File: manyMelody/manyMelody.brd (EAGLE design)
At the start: 74.9 x 95.2 mm, 13 parts, among them IC1 788TV

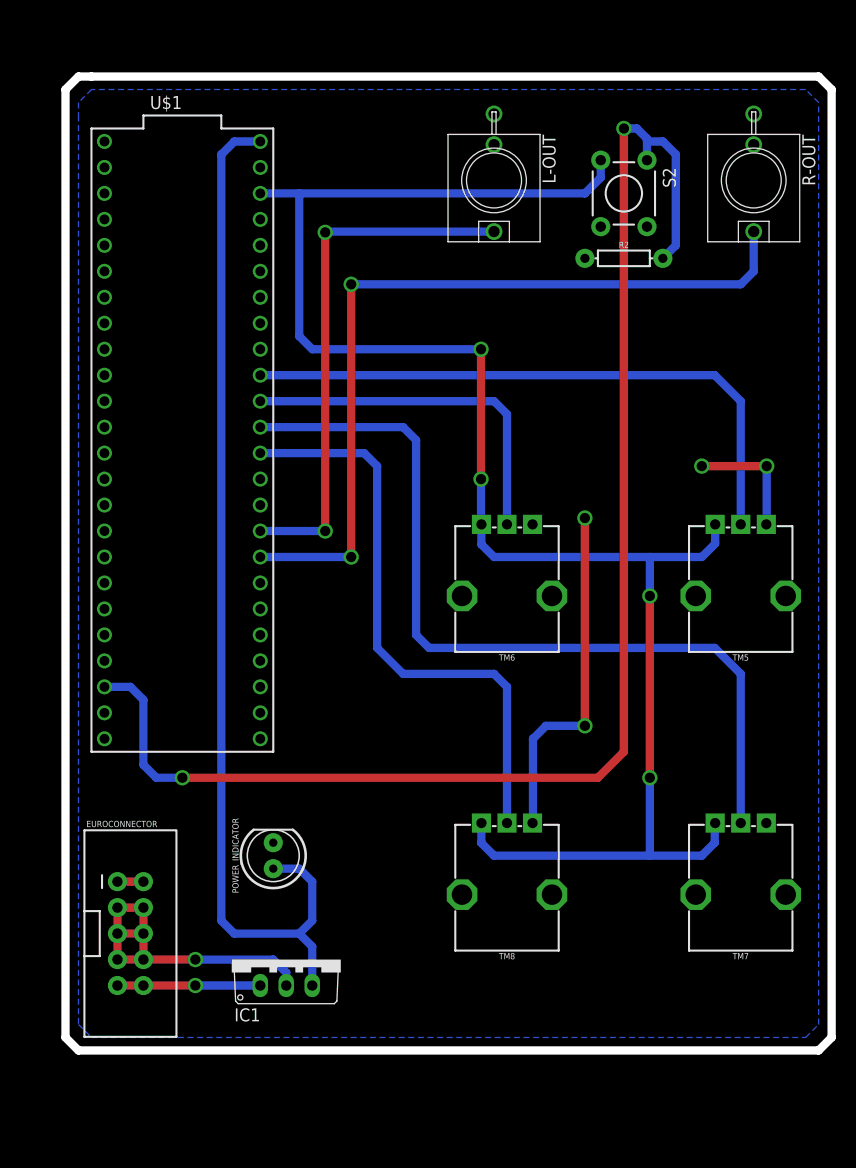
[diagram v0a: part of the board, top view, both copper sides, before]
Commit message: updated README
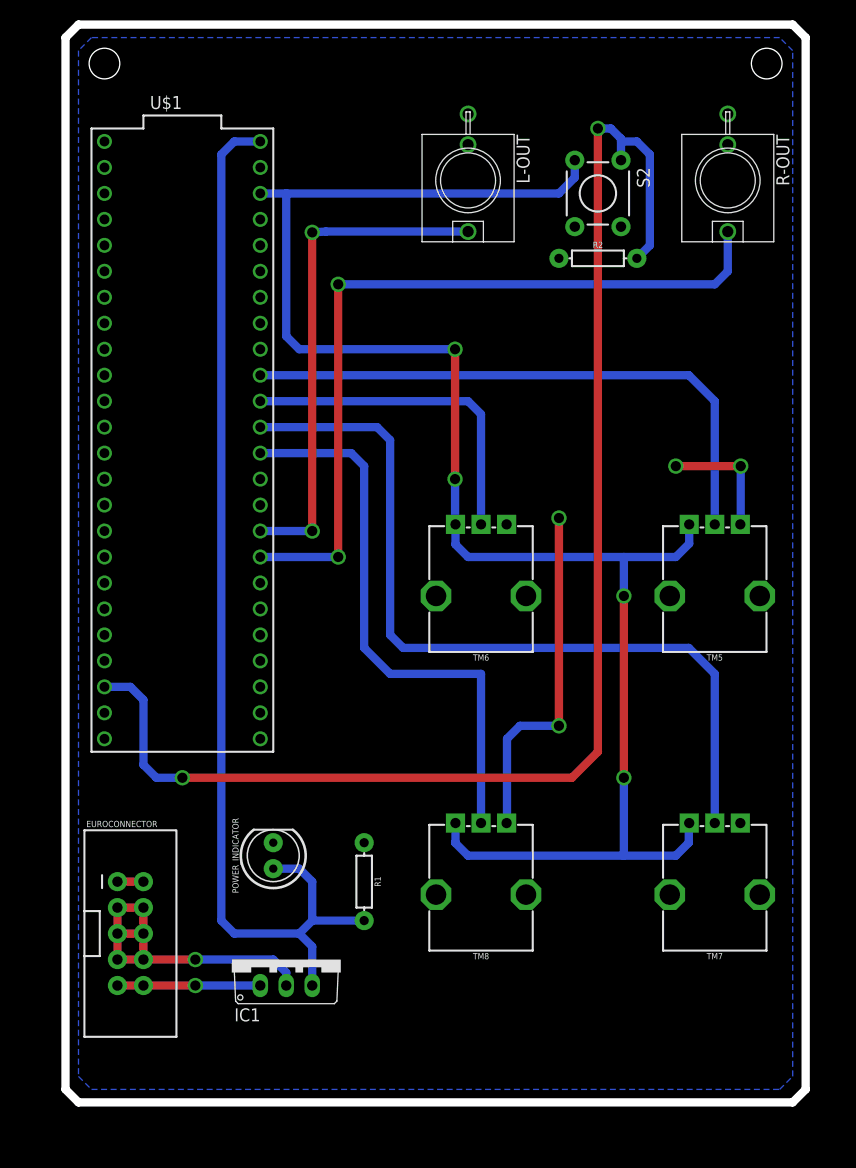
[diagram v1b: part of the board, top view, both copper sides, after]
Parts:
- added R1: 1k, SparkFun-Resistors:AXIAL-0.3
- moved L-OUT 2.54 mm to (86.4, 99.1)
- moved TM5 2.54 mm to (110.5, 58.4)
- moved TM6 2.54 mm to (87.6, 58.4)
- moved TM7 2.54 mm to (110.5, 29.2)
- moved TM8 2.54 mm to (87.6, 29.2)
- moved R-OUT 2.54 mm to (111.8, 99.1)
- moved R2 2.54 mm to (99.1, 91.4)
- moved S2 2.54 mm to (99.1, 97.8)
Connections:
- net 5V: now also R1.P$2
- net GND: now also R1.P$1
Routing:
- net 5V: track 103.0 -> 108.0 mm
- net 3.3V: track 169.8 -> 166.0 mm
- net N$9: track 52.1 -> 49.5 mm
- net N$13: track 35.4 -> 32.9 mm
- net N$14: track 60.1 -> 57.6 mm
- net N$12: track 82.7 -> 80.2 mm
- net N$10: track 79.3 -> 76.8 mm
- net N$3: track 139.0 -> 136.5 mm
- net N$11: track 57.3 -> 55.5 mm
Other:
- board size 74.9 x 95.2 mm -> 72.4 x 105.4 mm
